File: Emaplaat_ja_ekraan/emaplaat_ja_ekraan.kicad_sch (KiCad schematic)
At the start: 27 parts, among them IC1 TPS54429PWPR, IC2 ESP32-S3-WROOM-2-N32R16V, IC3 FT232RNL-TUBE, J1 Barrel_Jack, J2 USB4216-03-A

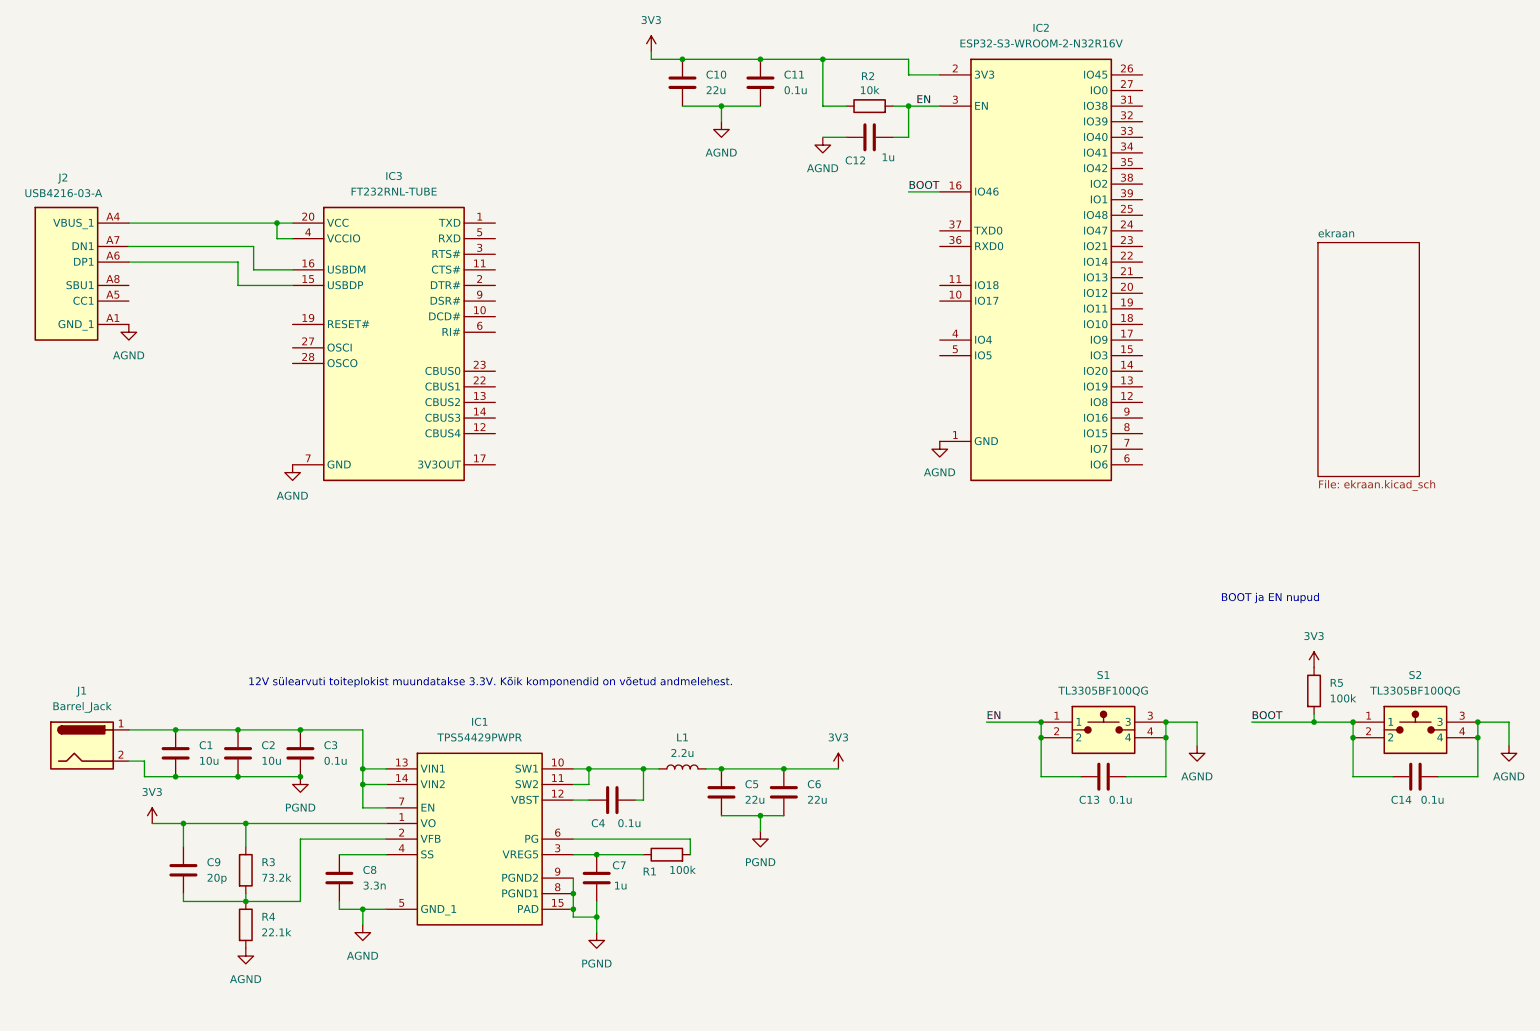
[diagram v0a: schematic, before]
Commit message: Urmas Tamm
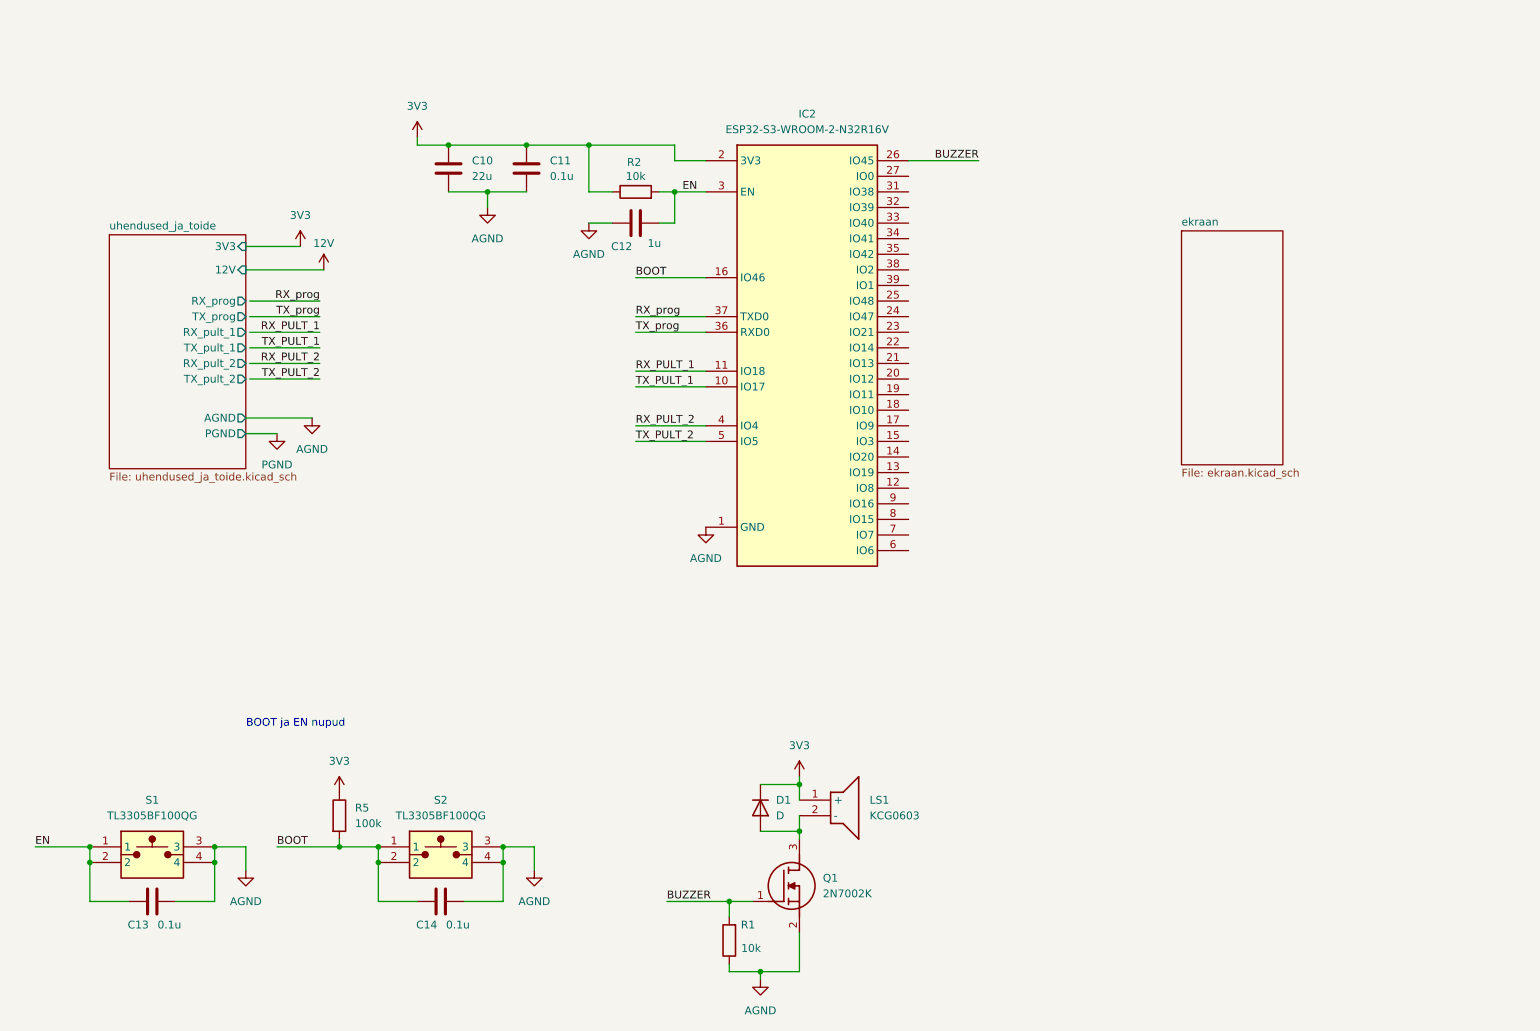
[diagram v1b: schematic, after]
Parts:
- removed C1, C2: 10u, symbol Device:C
- removed C3, C4: 0.1u, symbol Device:C
- removed C5, C6: 22u, symbol Device:C
- removed C7: 1u, symbol Device:C
- removed C8: 3.3n, symbol Device:C
- removed C9: 20p, symbol Device:C
- removed IC1: TPS54429PWPR, SOP65P640X120-15N, symbol TPS54429PWPR:TPS54429PWPR
- removed IC3: FT232RNL-TUBE, SOP65P780X200-28N, symbol FT232RNL-TUBE:FT232RNL-TUBE
- removed J1: Barrel_Jack, symbol Connector:Barrel_Jack
- removed J2: USB4216-03-A, USB421603A, symbol USB4216-03-A:USB4216-03-A
- removed L1: 2.2u, symbol Device:L
- removed R3: 73.2k, symbol Device:R
- removed R4: 22.1k, symbol Device:R
- added D1: D, symbol Device:D
- added LS1: KCG0603, KCG0603, symbol KCG0603:KCG0603
- added Q1: 2N7002K, SOT95P240X120-3N, symbol 2N7002K:2N7002K
- R1: value 100k -> 10k
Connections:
- net 3V3: now also D1.1 (K), LS1.1 (+)
- net AGND: now also R1.1, Q1.2 (S)
- net BUZZER: now reaches R1.2
- net BUZZER: now also IC2.26 (IO45), Q1.1 (G)
- net TX_PULT_1: now reaches IC2.10 (IO17)
- net RX_PULT_1: now reaches IC2.11 (IO18)
- net TX_prog: now reaches IC2.36 (RXD0)
- net RX_prog: now reaches IC2.37 (TXD0)
- net RX_PULT_2: now reaches IC2.4 (IO4)
- net TX_PULT_2: now reaches IC2.5 (IO5)
- new net: D1.2 (A), LS1.2 (-), Q1.3 (D)
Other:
- added sheet uhendused_ja_toide (uhendused_ja_toide.kicad_sch)
- note removed: "12V sülearvuti toiteplokist muundatakse 3.3V. Kõik komponendid on võetud andmelehest."
- moved on the sheet: C10, C11, C12, C13, C14, IC2, R2, R5, S1, S2
